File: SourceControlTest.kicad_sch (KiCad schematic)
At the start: 3 parts

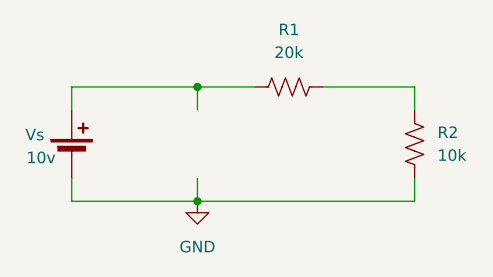
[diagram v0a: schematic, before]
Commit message: Revert "deleted capacitor"
This reverts commit d5b02636a01619e9b602a21c2b5c62289a5c960a.
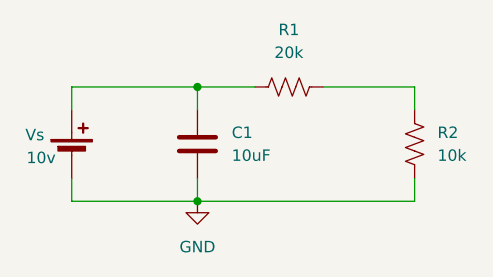
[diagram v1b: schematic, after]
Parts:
- added C1: 10uF, symbol Device:C
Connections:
- net GND: now also C1.2
- net at R1.1, Vs.1 (+): now also C1.1
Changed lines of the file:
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@@
+	)
+	(symbol
+		(lib_id "Device:C")
+		(at 128.27 95.25 0)
+		(unit 1)
+		(body_style 1)
+		(exclude_from_sim no)
+		(in_bom yes)
+		(on_board yes)
+		(in_pos_files yes)
+		(dnp no)
+		(fields_autoplaced yes)
+		(property "Reference" "C1"
+			(at 132.08 93.9799 0)
+			(show_name no)
+			(do_not_autoplace no)
+			(effects
+				(font
+					(size 1.27 1.27)
+				)
+				(justify left)
+			)
+		)
+		(property "Value" "10uF"
+			(at 132.08 96.5199 0)
+			(show_name no)
+			(do_not_autoplace no)
+			(effects
+				(font
+					(size 1.27 1.27)
+				)
+				(justify left)
+			)
+		)
+		(property "Footprint" ""
+			(at 129.2352 99.06 0)
+			(hide yes)
+			(show_name no)
+			(do_not_autoplace no)
+			(effects
+				(font
+					(size 1.27 1.27)
+				)
+			)
+		)
+		(property "Datasheet" ""
+			(at 128.27 95.25 0)
+			(hide yes)
+			(show_name no)
+			(do_not_autoplace no)
+			(effects
+				(font
+					(size 1.27 1.27)
+				)
+			)
+		)
+		(property "Description" "Unpolarized capacitor"
+			(at 128.27 95.25 0)
+			(hide yes)
+			(show_name no)
+			(do_not_autoplace no)
+			(effects
+				(font
+					(size 1.27 1.27)
+				)
+			)
+		)
+		(pin "2"
+		)
+		(pin "1"
+		)
+		(instances
+			(project "SourceControlTest"
+				(path "/5d981c2c-ab3d-4850-ba6d-abf03e2cd683"
+					(reference "C1")
+					(unit 1)
+				)
+			)
+		)
 	)
 	(symbol
